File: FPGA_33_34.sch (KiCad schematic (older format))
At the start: 14 parts, among them U1 XC7K160T-FFG676, U42 TXB0108PW

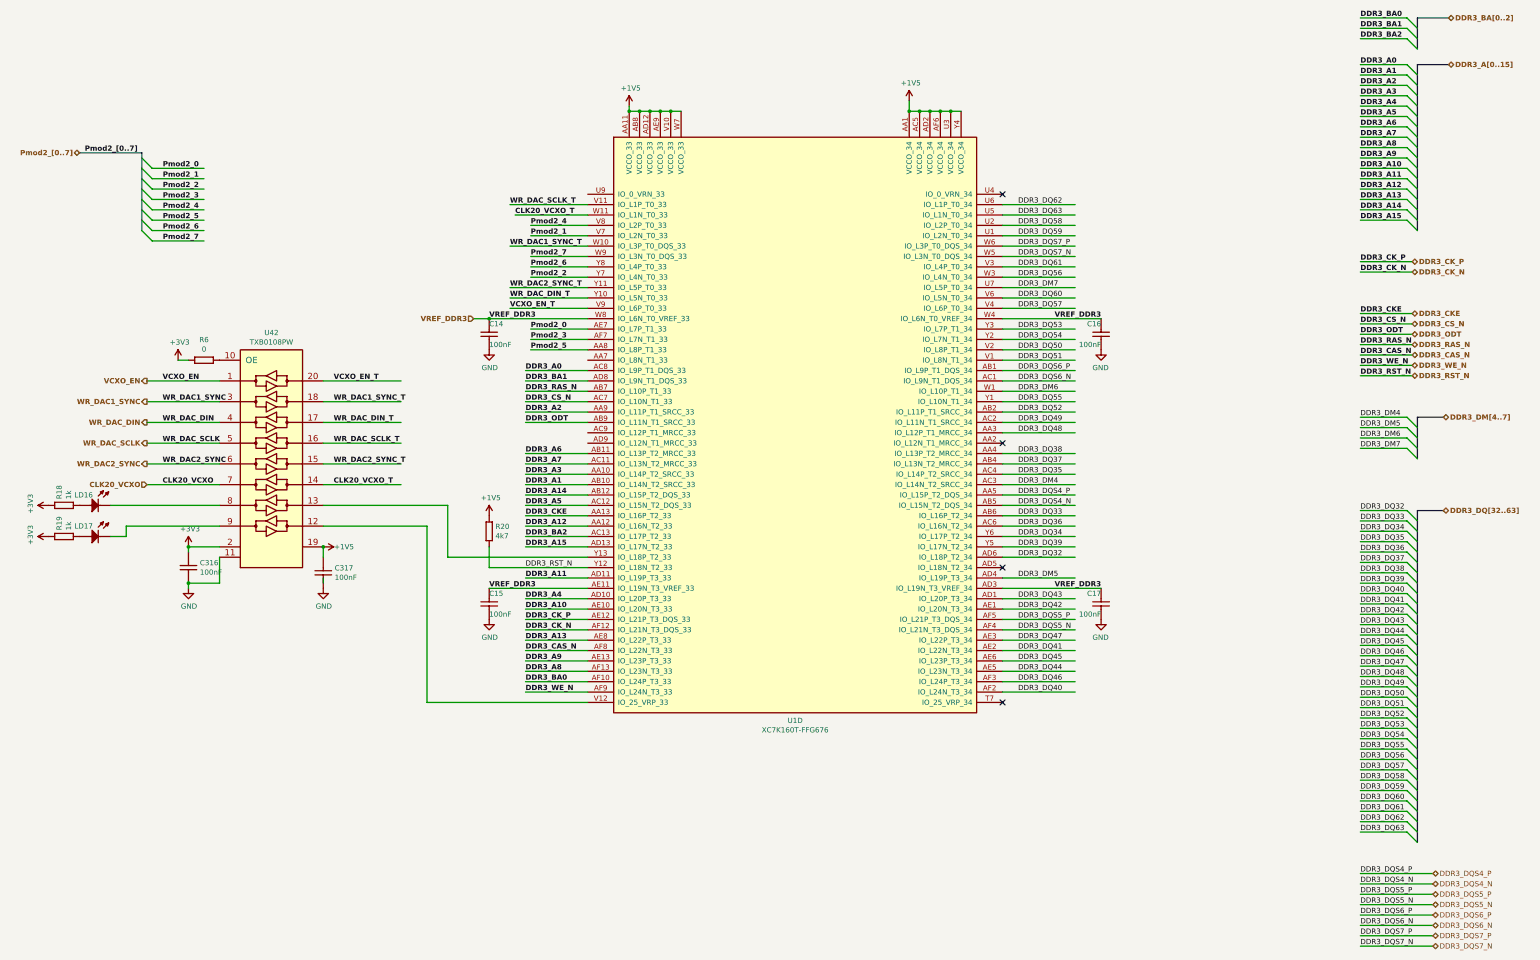
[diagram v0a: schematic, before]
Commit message: REF CLK for MIG
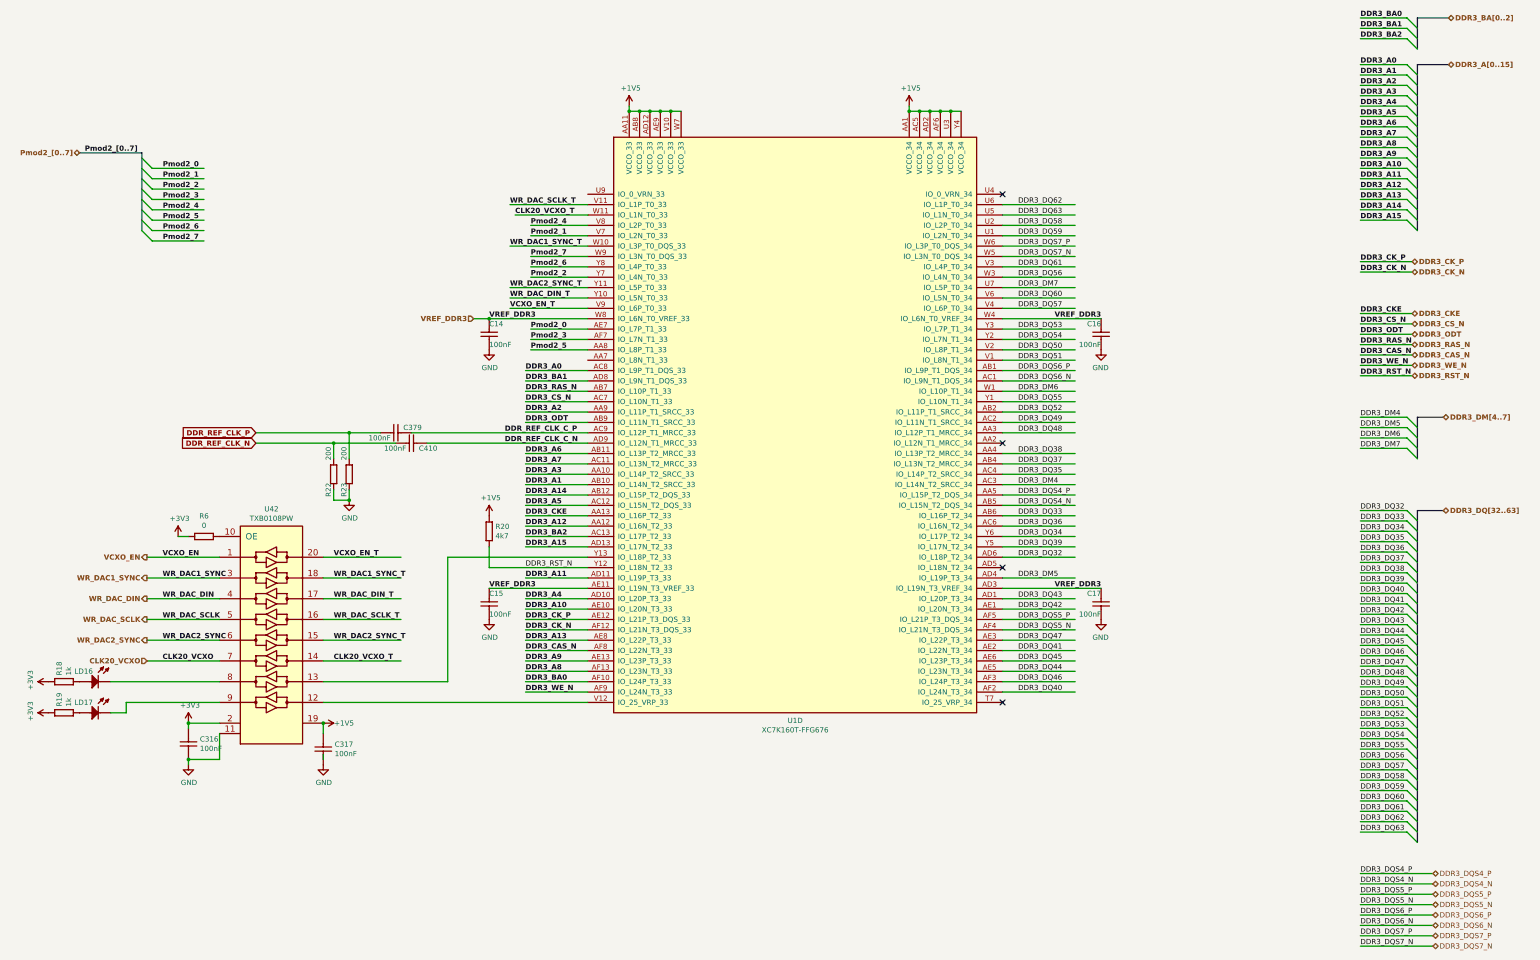
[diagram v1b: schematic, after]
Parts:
- added C379, C410: CC0201_100NF_6.3V_10%_X5R, CAPC0603X33N, symbol Capacitors_SMD:CC0201_100NF_6.3V_10%_X5R
- added R22, R23: R0201_100R_1%_0.05W_200PPM, RESC0603X28N, symbol Resistors_SMD:R0201_100R_1%_0.05W_200PPM
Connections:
- net labels added: DDR_REF_CLK_C_N, DDR_REF_CLK_C_P, DDR_REF_CLK_N, DDR_REF_CLK_P
- wire segments 214 -> 223
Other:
- moved on the sheet: C316, C317, LD16, LD17, R18, R19, R6, U42
